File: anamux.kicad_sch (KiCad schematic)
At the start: 3 parts, among them J51 Conn_02x08_Odd_Even, U26 CD4051B

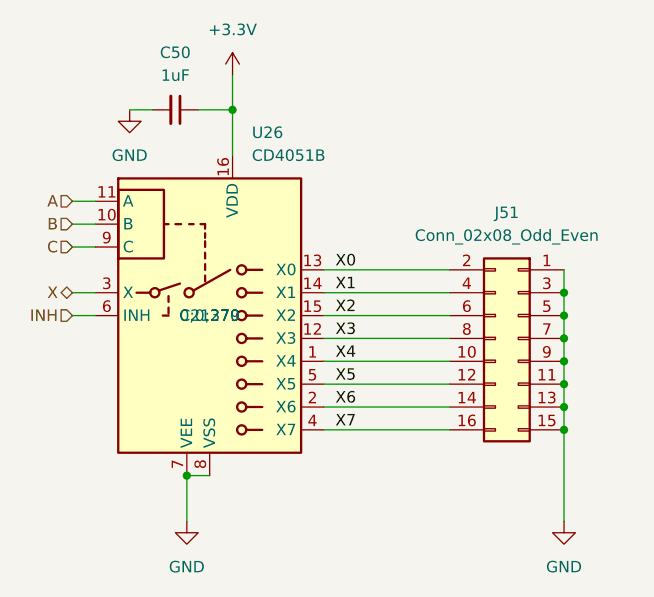
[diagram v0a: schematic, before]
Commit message: WIP v0.2.0 changes
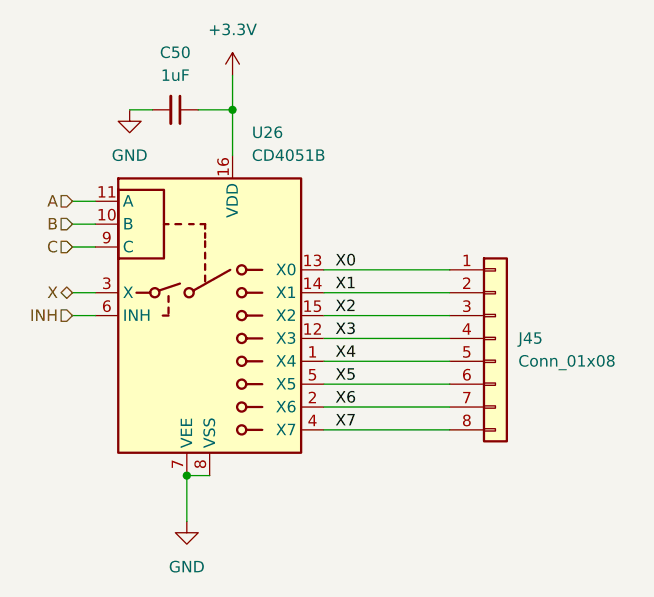
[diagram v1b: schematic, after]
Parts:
- J45: renamed from J51; value Conn_02x08_Odd_Even -> Conn_01x08; footprint HL_Connector_Pad_2.54mm:Pad_2x08_P2.54_1.7x1.7_Rect-Oct -> HL_Connector_Pad_2.54mm:Pad_1x08_P2.54_1.7x1.7_Oct; symbol Connector_Generic:Conn_02x08_Odd_Even -> Connector_Generic:Conn_01x08
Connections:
- net GND: no longer J45.1 (Pin_1), J45.11 (Pin_11), J45.13 (Pin_13), J45.15 (Pin_15), J45.3 (Pin_3), J45.5 (Pin_5), J45.7 (Pin_7), J45.9 (Pin_9)
- net X0: now also J45.1 (Pin_1); no longer J45.2 (Pin_2)
- net X1: now also J45.2 (Pin_2); no longer J45.4 (Pin_4)
- net X2: now also J45.3 (Pin_3); no longer J45.6 (Pin_6)
- net X3: now also J45.4 (Pin_4); no longer J45.8 (Pin_8)
- net X4: now also J45.5 (Pin_5); no longer J45.10 (Pin_10)
- net X5: now also J45.6 (Pin_6); no longer J45.12 (Pin_12)
- net X6: now also J45.7 (Pin_7); no longer J45.14 (Pin_14)
- net X7: now also J45.8 (Pin_8); no longer J45.16 (Pin_16)
